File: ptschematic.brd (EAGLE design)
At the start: 100 x 80 mm, 28 parts, among them U3 NCP1117LPST33T3G, U4 BGM13S, Y2 32MHz

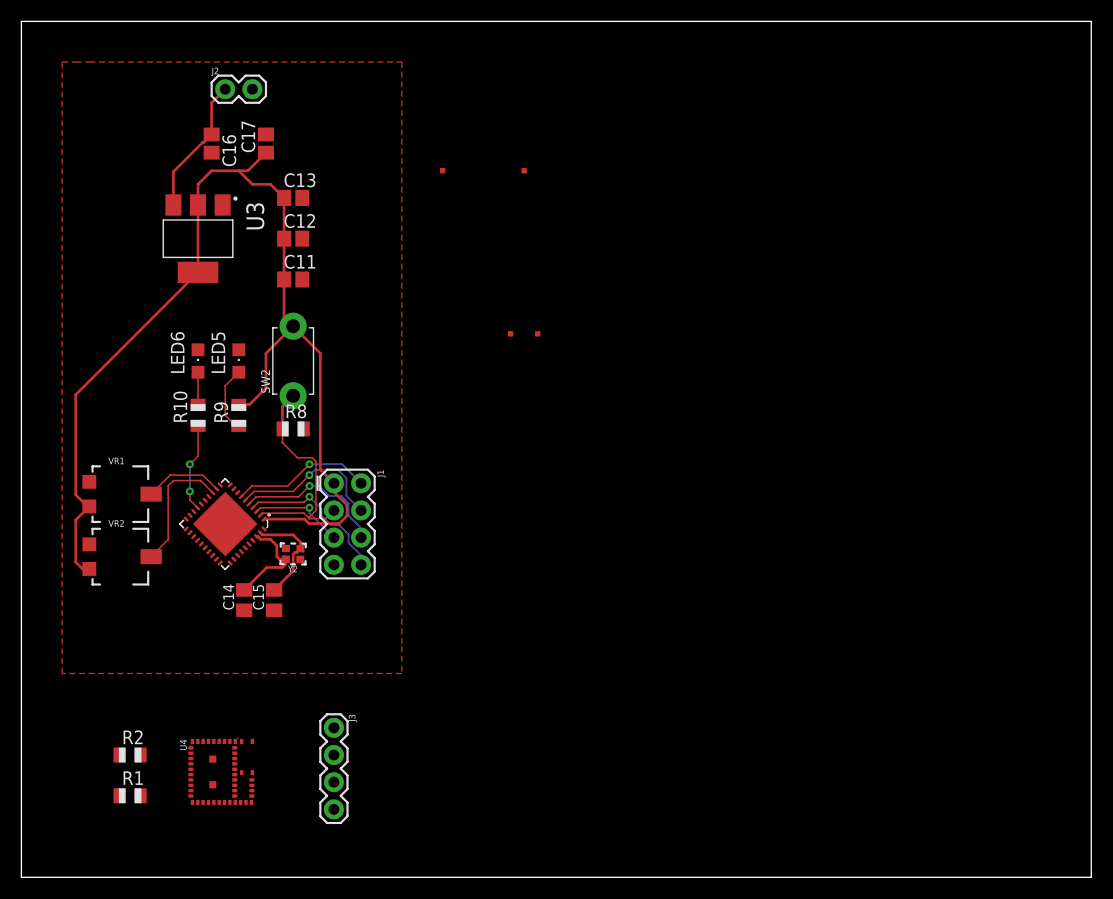
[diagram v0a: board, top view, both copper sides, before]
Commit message: finished tracing BGM
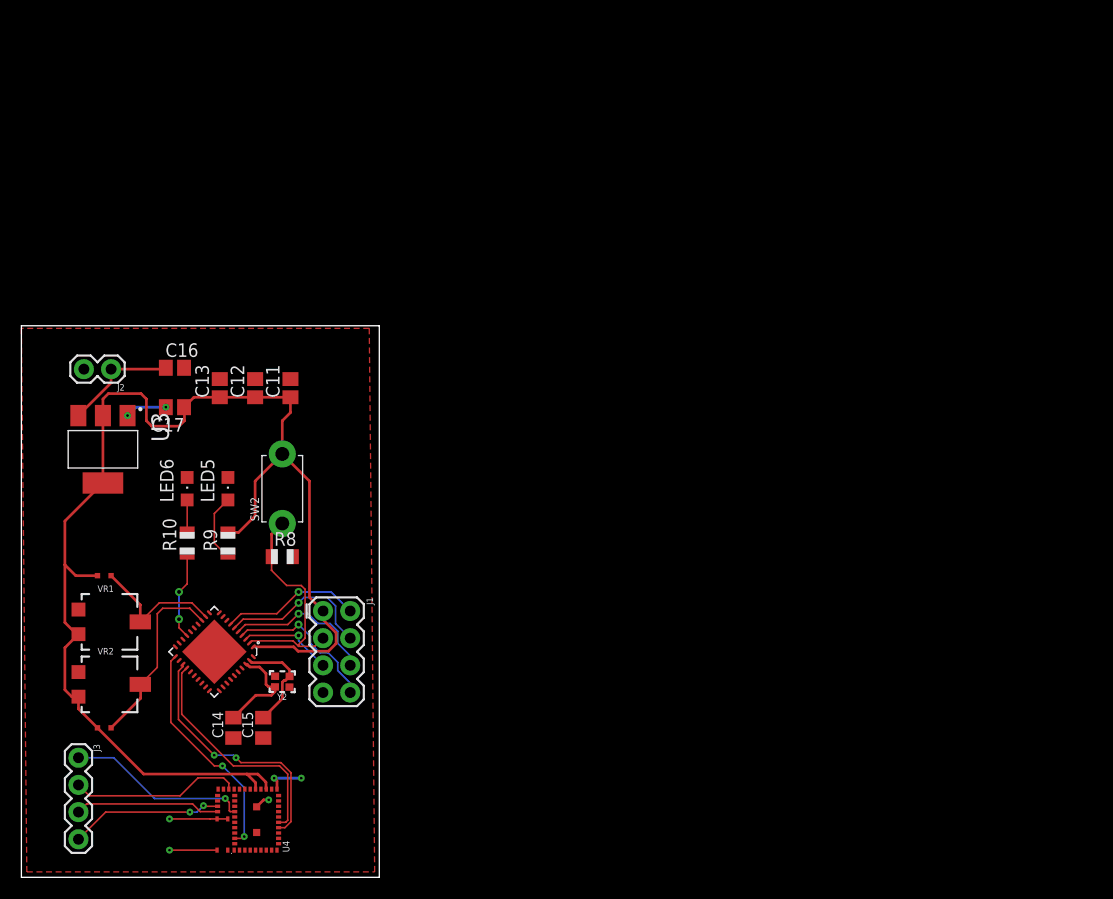
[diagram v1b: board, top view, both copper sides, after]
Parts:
- removed R1, R2: 0, adafruit:R0805
- moved TP3 60.6 mm to (8.38, 14.0)
- moved TP1 55.2 mm to (7.11, 14.0)
- moved TP4 54.1 mm to (8.38, 28.2)
- moved TP2 44.7 mm to (7.11, 28.2)
- moved J2 28.3 mm to (8.38, 47.5), turned to 180 degrees
- moved C17 26.1 mm to (14.4, 43.9), turned to 180 degrees
- moved J3 24.0 mm to (5.33, 11.2)
- moved U3 21.6 mm to (7.62, 40.0)
- moved C16 21.2 mm to (14.4, 47.6), turned to 0 degrees
- moved C13 19.1 mm to (18.5, 45.7), turned to 90 degrees
- moved C12 14.4 mm to (21.8, 45.7), turned to 90 degrees
- moved J1 12.0 mm to (29.5, 21.1)
- moved U$1 12.0 mm to (18.0, 21.1)
- moved VR2 12.0 mm to (7.87, 18.0)
- moved C14 12.0 mm to (19.8, 14.0)
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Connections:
- removed net ANT_GND: U4.P$47
- removed net N$5: R1.2, U4.P$2
- removed net N$6: R1.1, R2.1, U4.P$3
- net ADC1: now also TP4.P$1
- net ADC2: now also TP3.P$1
- net GND: now also U4.P$2, U4.P$3, U4.P$47; no longer R2.2, TP3.P$1, TP4.P$1
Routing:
- net A1RXD: track 0.00 -> 23.9 mm, vias 0 -> 2
- net A1TXD: track 0.00 -> 22.0 mm
- net BGMRST: track 0.00 -> 21.2 mm, vias 0 -> 2
- net GND: track 0.00 -> 18.9 mm, vias 0 -> 7
- net N$4: track 0.00 -> 17.1 mm, vias 0 -> 1
- net 3.3V: track 107.3 -> 124.5 mm
- net N$3: track 0.00 -> 15.9 mm
- net N$1: track 0.00 -> 14.3 mm, vias 0 -> 2
- net N$2: track 0.00 -> 13.6 mm
- net ADC1: track 7.38 -> 12.8 mm
- net ADC2: track 12.1 -> 17.4 mm
- net VIN: track 12.9 -> 10.8 mm
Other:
- board size 100 x 80 mm -> 33.5 x 51.6 mm
